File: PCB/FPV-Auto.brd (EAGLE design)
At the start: 65.5 x 30 mm, 97 parts, among them Q310 CSD25402Q3A, Q320 BSS138, U100 ATMEGA328P-AU, U110 NRF24L01+_MINI, U120 74LVC2T45DCT, U140 DRV8835, U200 RASPBERRY_PI_ZERO_W_V1.1_GPIO, U210 MAX98357A, U300 BQ25892, U330 TPS61236P, U340 TPS61236P, U350 LP5907MFX-3.3/NOPB, X100 ISP-M_TP, X120 M06_2X03R, X140 M04_2X03R, X210 M02_2X01L, X320 M02_2X01L, X340 M02_2X01L, Y100 8Mhz

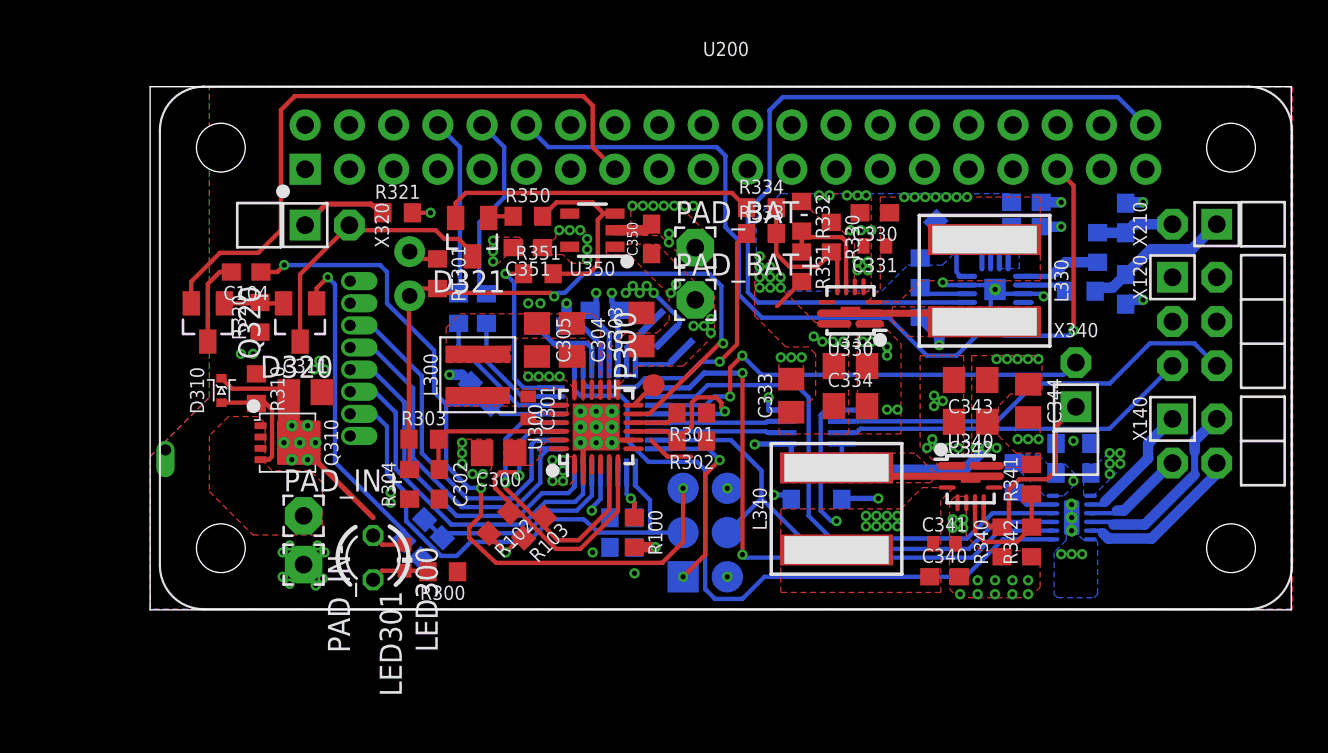
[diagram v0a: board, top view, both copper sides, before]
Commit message: Updated PCB
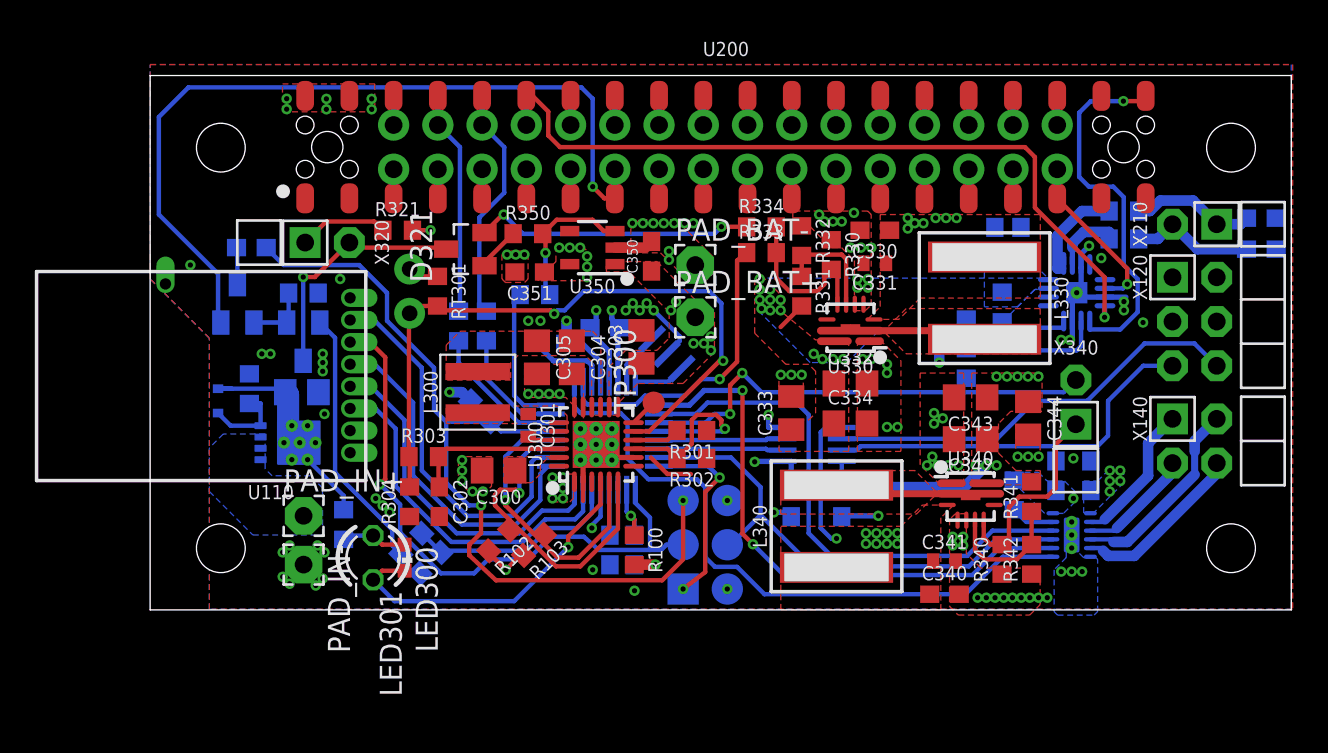
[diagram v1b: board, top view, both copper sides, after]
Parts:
- added U$3: (no value), FPV-Auto:HACKFFM_LOGO_STOP
- added U$9: (no value), FPV-Auto:DATE
- U200: value RASPBERRY_PI_ZERO_W_V1.1_GPIO -> RASPBERRY_PI_ZERO_W_V1.1_GPIO_DUAL; device FPV-Auto:RASPBERRY_PI_ZERO_W_V1.1_GPIO -> FPV-Auto:RASPBERRY_PI_ZERO_W_V1.1_GPIO_DUAL
- moved C212 8.13 mm to (63.8, 20.7), turned to 180 degrees
- moved C213 7.79 mm to (63.8, 22.5), turned to 180 degrees
- moved R300 6.30 mm to (11.1, 4.90), flipped to the bottom, turned to 90 degrees
- moved R210 5.37 mm to (48.9, 17.4), turned to 90 degrees
- moved U210 4.69 mm to (53.2, 18.2), turned to 90 degrees
- moved R211 4.39 mm to (46.9, 15.0)
- moved FB211 3.91 mm to (55.9, 21.3)
- moved C210 2.92 mm to (48.5, 21.1), turned to 90 degrees
- moved R320 2.85 mm to (8.80, 18.2), flipped to the bottom, turned to 0 degrees
- moved FB210 2.58 mm to (55.9, 22.9), turned to 180 degrees
- moved Q320 2.02 mm to (5.01, 17.6), flipped to the bottom, turned to 90 degrees
- moved C104 1.43 mm to (5.81, 20.8), flipped to the bottom, turned to 0 degrees
- moved C351 1.40 mm to (21.8, 19.4)
- moved R332 1.40 mm to (37.4, 21.2)
- moved R331 1.40 mm to (37.4, 18.3)
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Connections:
- removed net NRF_CE: U100.26, U110.3
- removed net NRF_MOSI: U100.23, U110.6
- removed net SCK/NRF_MISO: U100.17, U110.7, X100.3
- new net NRF_CS: U100.23, U110.3
- new net NRF_MISO: U100.26, U110.7
- new net SCK/NRF_MOSI: U100.17, U110.6, X100.3
- net +5V1: now also U200.SMD_2, U200.SMD_4; no longer U200.2, U200.4
- net BCLK: now also U200.SMD_12
- net DIN: now also U200.SMD_40; no longer U200.40
- net GND: now also U200.SMD_14, U200.SMD_20, U200.SMD_25, U200.SMD_30, U200.SMD_34, U200.SMD_39, U200.SMD_6, U200.SMD_9; no longer U200.39
- net LRCLK: now also U200.SMD_35
- net N$15: now also D320.2; no longer D320.1
- net N$18: now also D320.1; no longer D320.2
- net N$26: now also U200.SMD_8
- net N$27: now also U200.SMD_10
- net NRF_!CS: now also U100.24; no longer U100.25
- net NRF_SCK: now also U100.25; no longer U100.24
- net RASPI_DTR: now also U200.SMD_15
- net VO+: now also X210.1; no longer X210.2
- net VO-: now also X210.2; no longer X210.1
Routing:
- net SCK/NRF_MOSI: track 0.00 -> 35.8 mm, vias 0 -> 1
- net SCK/NRF_MISO: track 30.5 -> 0.00 mm
- net DIN: track 46.3 -> 21.5 mm, vias 0 -> 1
- net NRF_MISO: track 0.00 -> 22.2 mm
- net NRF_CE: track 20.8 -> 0.00 mm
- net NRF_CS: track 0.00 -> 20.5 mm
- net NRF_MOSI: track 20.4 -> 0.00 mm
- net N$19: track 3.41 -> 19.5 mm, vias 0 -> 1
- net RASPI_DTR: track 37.2 -> 47.4 mm, vias 0 -> 1
- net BCLK: track 37.6 -> 44.7 mm, vias 0 -> 1
- net GND: track 44.6 -> 38.9 mm, vias 108 -> 113
- net GAIN: track 2.82 -> 8.17 mm
- net LRCLK: track 14.9 -> 9.64 mm
- net N$15: track 18.7 -> 15.2 mm, vias 1 -> 0
- net DTR: track 4.95 -> 2.15 mm
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- added copper zone on layer 15, net GND
- added copper zone on layer 16, net INPUT
- removed copper zone on layer 1, net INPUT
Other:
- board size 65.5 x 30 mm -> 65.5 x 30.7 mm
- board text removed: "MotA MotB"
- board text removed: "Servo1 Servo2"
